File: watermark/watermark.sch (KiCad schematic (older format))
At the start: 7 parts

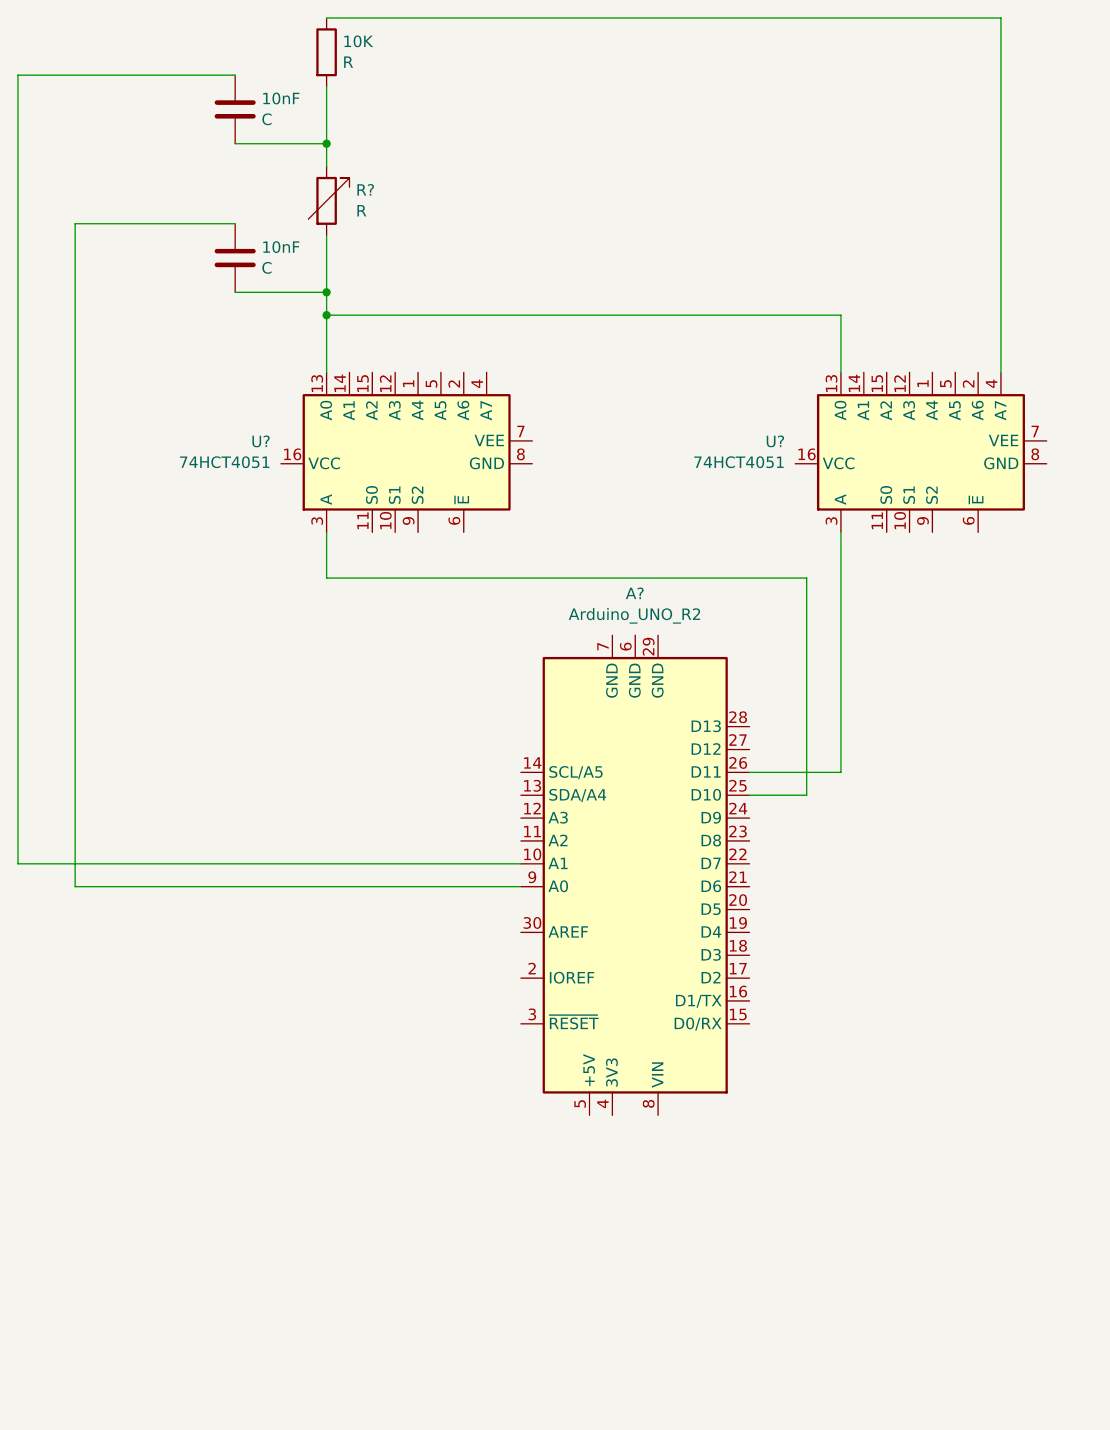
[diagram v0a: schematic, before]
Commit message: m
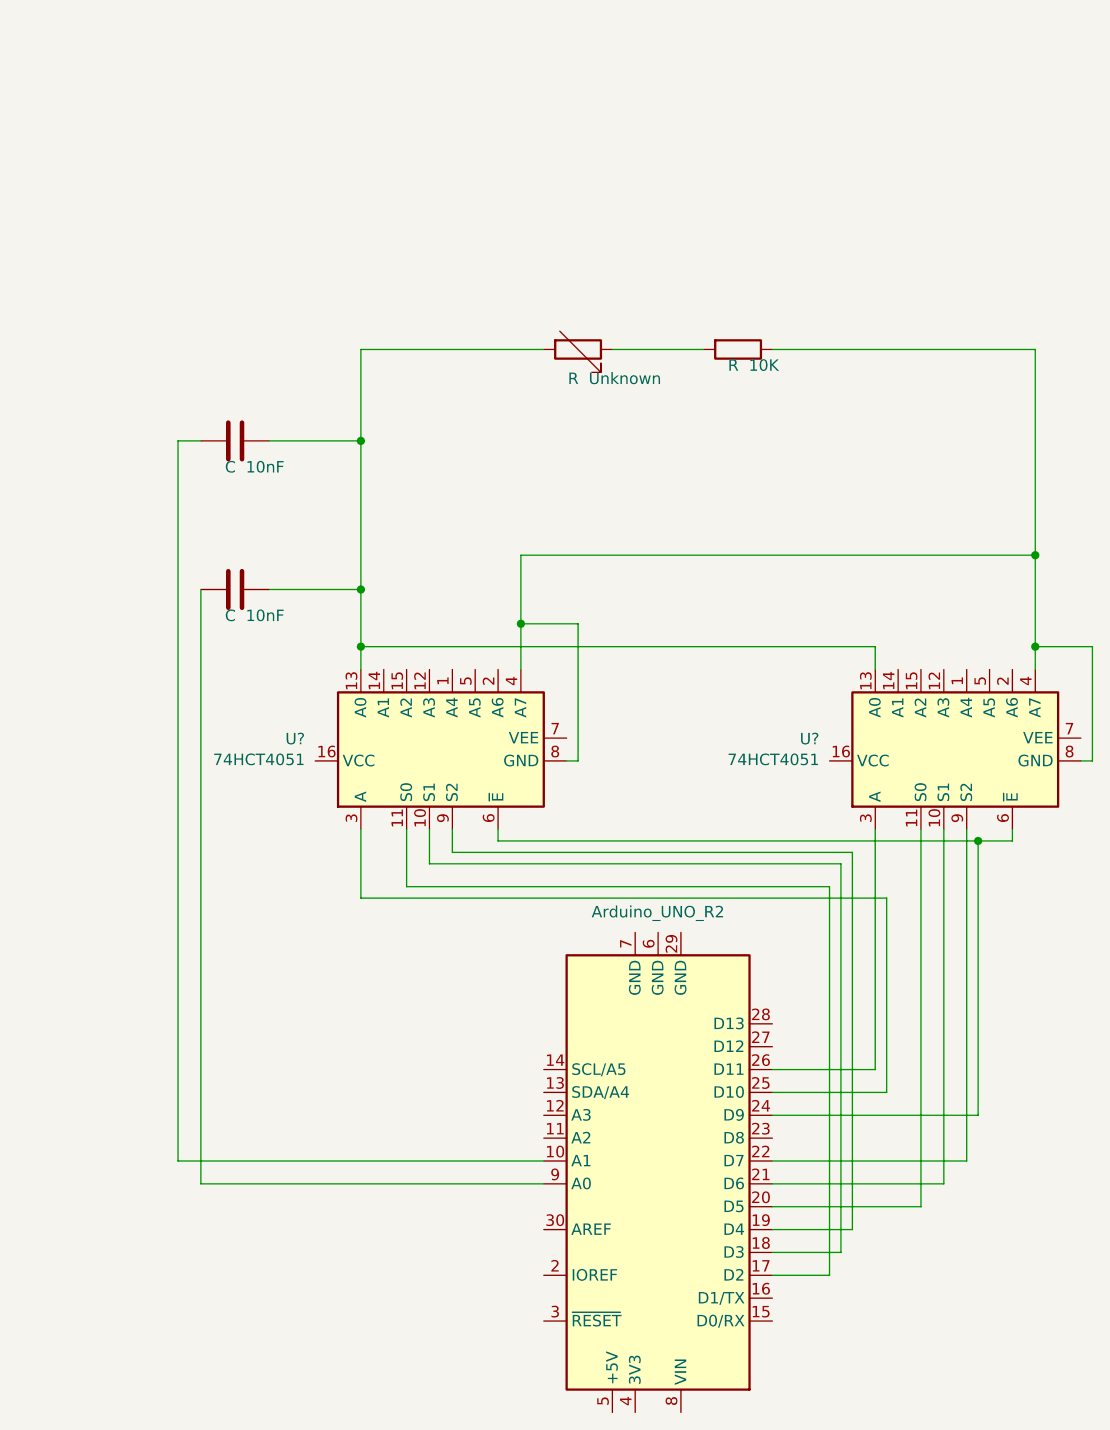
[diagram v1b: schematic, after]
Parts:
- gave numbers to parts that had none: 1
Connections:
- net at U?.10 (S1): now also A?.21 (D6)
- net at U?.11 (S0): now also A?.20 (D5)
- net at U?.13 (A0), U?.13 (A0), Unknown.2: now also 10nF.1, 10nF.1; no longer 10nF.2
- net at 10K.1, U?.4 (A7): now also U?.4 (A7), U?.8 (GND), U?.8 (GND)
- net at U?.6 (~E): now also A?.24 (D9), U?.6 (~E)
- net at U?.9 (S2): now also A?.22 (D7)
- net at U?.10 (S1): now also A?.18 (D3)
- net at U?.11 (S0): now also A?.17 (D2)
- net at U?.9 (S2): now also A?.19 (D4)
- net at 10K.2, Unknown.1: no longer 10nF.2
- net at A?.10 (A1): now also 10nF.2; no longer 10nF.1
- net at A?.9 (A0): now also 10nF.2; no longer 10nF.1
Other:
- moved on the sheet: 10K, 10nF, U?, Unknown
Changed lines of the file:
@@
 $EndDescr
+$Comp
+L Device:R_Variable Unknown
+U 1 1 608B5481
+P 4050 2900
+F 0 "Unknown" V 4178 2946 50  0000 L CNN
+F 1 "R" V 4178 2855 50  0000 L CNN
+F 2 "" V 3980 2900 50  0001 C CNN
+F 3 "~" H 4050 2900 50  0001 C CNN
+	1    4050 2900
+	0    1    1    0
+$EndComp
+$Comp
+L Device:R 10K
+U 1 1 608B5D06
+P 4750 2900
+F 0 "10K" V 4820 2946 50  0000 L CNN
+F 1 "R" V 4820 2855 50  0000 L CNN
+F 2 "" V 4680 2900 50  0001 C CNN
+F 3 "~" H 4750 2900 50  0001 C CNN
+	1    4750 2900
+	0    1    1    0
+$EndComp
+$Comp
+L Device:C 10nF
+U 1 1 608C2E1E
+P 2550 3950
+F 0 "10nF" V 2665 3996 50  0000 L CNN
+F 1 "C" V 2665 3905 50  0000 L CNN
+F 2 "" H 2588 3800 50  0001 C CNN
+F 3 "~" H 2550 3950 50  0001 C CNN
+	1    2550 3950
+	0    1    1    0
+$EndComp
+$Comp
+L Device:C 10nF
+U 1 1 608C5621
+P 2550 3300
+F 0 "10nF" V 2665 3346 50  0000 L CNN
+F 1 "C" V 2665 3255 50  0000 L CNN
+F 2 "" H 2588 3150 50  0001 C CNN
+F 3 "~" H 2550 3300 50  0001 C CNN
+	1    2550 3300
+	0    1    1    0
+$EndComp
+Wire Wire Line
+	3100 5300 3100 5000
+Wire Wire Line
+	3300 5250 3300 5000
+Wire Wire Line
+	3400 5150 3400 5000
+Wire Wire Line
+	5200 5150 3400 5150
+Wire Wire Line
+	4050 4700 4000 4700
+Wire Wire Line
+	5400 5300 3100 5300
+Wire Wire Line
+	5800 5050 5950 5050
+$Comp
+L MCU_Module:Arduino_UNO_R2 A?
+U 1 1 608BD114
+P 4400 6550
+F 0 "A?" H 4400 5269 50  0001 C CNN
+F 1 "Arduino_UNO_R2" H 4400 5361 50  0000 C CNN
+F 2 "Module:Arduino_UNO_R2" H 4400 6550 50  0001 C CIN
+F 3 "https://www.arduino.cc/en/Main/arduinoBoardUno" H 4400 6550 50  0001 C CNN
+	1    4400 6550
+	-1   0    0    1
+$EndComp
+Wire Wire Line
+	4900 6150 5400 6150
+Wire Wire Line
+	5400 6150 5400 5300
+Wire Wire Line
+	4900 6050 5350 6050
+Wire Wire Line
+	5800 5050 5800 6250
+Wire Wire Line
+	4900 6450 5750 6450
+Wire Wire Line
+	4900 6550 5650 6550
+Wire Wire Line
+	4900 6750 5250 6750
+Wire Wire Line
+	4900 6850 5200 6850
+Wire Wire Line
+	5800 6250 4900 6250
+Wire Wire Line
+	5200 6850 5200 5150
+Wire Wire Line
+	5150 5250 3300 5250
+Wire Wire Line
+	4900 6950 5150 6950
+Wire Wire Line
+	5150 6950 5150 5250
+Wire Wire Line
+	5750 6450 5750 5000
+Wire Wire Line
+	5950 5050 5950 5000
+Wire Wire Line
+	5350 6050 5350 5000
+Wire Wire Line
+	5650 6550 5650 5000
 $Comp
 L 74xx:74HCT4051 U?
 U 1 1 608AFB59
-P 5500 3400
-F 0 "U?" V 5596 3944 50  0000 L CNN
-F 1 "74HCT4051" V 5505 3944 50  0000 L CNN
-F 2 "" H 5500 3000 50  0001 C CNN
-F 3 "http://www.ti.com/lit/ds/symlink/cd74hct4051.pdf" H 5500 3000 50  0001 C CNN
-	1    5500 3400
+P 5650 4700
+F 0 "U?" V 5746 5244 50  0000 L CNN
+F 1 "74HCT4051" V 5655 5244 50  0000 L CNN
+F 2 "" H 5650 4300 50  0001 C CNN
+F 3 "http://www.ti.com/lit/ds/symlink/cd74hct4051.pdf" H 5650 4300 50  0001 C CNN
+	1    5650 4700
 	0    -1   -1   0
 $EndComp
+Wire Wire Line
+	5550 5000 5550 6650
+Wire Wire Line
+	5550 6650 4900 6650
 $Comp
 L 74xx:74HCT4051 U?
 U 1 1 608B37CA
-P 3250 3400
-F 0 "U?" V 3346 3944 50  0000 L CNN
-F 1 "74HCT4051" V 3255 3944 50  0000 L CNN
-F 2 "" H 3250 3000 50  0001 C CNN
-F 3 "http://www.ti.com/lit/ds/symlink/cd74hct4051.pdf" H 3250 3000 50  0001 C CNN
-	1    3250 3400
+P 3400 4700
+F 0 "U?" V 3496 5244 50  0000 L CNN
+F 1 "74HCT4051" V 3405 5244 50  0000 L CNN
+F 2 "" H 3400 4300 50  0001 C CNN
+F 3 "http://www.ti.com/lit/ds/symlink/cd74hct4051.pdf" H 3400 4300 50  0001 C CNN
+	1    3400 4700
 	0    -1   -1   0
 $EndComp
-$Comp
-L Device:R_Variable R?
-U 1 1 608B5481
-P 2950 2250
-F 0 "R?" H 3078 2296 50  0000 L CNN
-F 1 "R" H 3078 2205 50  0000 L CNN
-F 2 "" V 2880 2250 50  0001 C CNN
-F 3 "~" H 2950 2250 50  0001 C CNN
-	1    2950 2250
-	1    0    0    -1
-$EndComp
-$Comp
-L Device:R 10K
-U 1 1 608B5D06
-P 2950 1600
-F 0 "10K" H 3020 1646 50  0000 L CNN
-F 1 "R" H 3020 1555 50  0000 L CNN
-F 2 "" V 2880 1600 50  0001 C CNN
-F 3 "~" H 2950 1600 50  0001 C CNN
-	1    2950 1600
-	1    0    0    -1
-$EndComp
-Wire Wire Line
-	2950 3000 2950 2750
-Wire Wire Line
-	2950 2100 2950 2000
-Wire Wire Line
-	2950 1450 5900 1450
-Wire Wire Line
-	5900 1450 5900 3000
-Wire Wire Line
-	5200 3000 5200 2750
-Wire Wire Line
-	5200 2750 2950 2750
-Connection ~ 2950 2750
-$Comp
-L MCU_Module:Arduino_UNO_R2 A?
-U 1 1 608BD114
-P 4300 5250
-F 0 "A?" H 4300 3969 50  0000 C CNN
-F 1 "Arduino_UNO_R2" H 4300 4060 50  0000 C CNN
-F 2 "Module:Arduino_UNO_R2" H 4300 5250 50  0001 C CIN
-F 3 "https://www.arduino.cc/en/Main/arduinoBoardUno" H 4300 5250 50  0001 C CNN
-	1    4300 5250
-	-1   0    0    1
-$EndComp
-Wire Wire Line
-	1850 5250 3800 5250
-Wire Wire Line
-	2950 2000 2550 2000
-Wire Wire Line
-	1600 5150 3800 5150
-Connection ~ 2950 2000
-Wire Wire Line
-	2950 2000 2950 1750
-$Comp
-L Device:C 10nF
-U 1 1 608C2E1E
-P 2550 2500
-F 0 "10nF" H 2665 2546 50  0000 L CNN
-F 1 "C" H 2665 2455 50  0000 L CNN
-F 2 "" H 2588 2350 50  0001 C CNN
-F 3 "~" H 2550 2500 50  0001 C CNN
-	1    2550 2500
-	1    0    0    -1
-$EndComp
-Wire Wire Line
-	2950 2400 2950 2650
-Wire Wire Line
-	2950 2650 2550 2650
-Connection ~ 2950 2650
-Wire Wire Line
-	2950 2650 2950 2750
-Wire Wire Line
-	2550 2350 1850 2350
-Wire Wire Line
-	1850 2350 1850 5250
-$Comp
-L Device:C 10nF
-U 1 1 608C5621
-P 2550 1850
-F 0 "10nF" H 2665 1896 50  0000 L CNN
-F 1 "C" H 2665 1805 50  0000 L CNN
-F 2 "" H 2588 1700 50  0001 C CNN
-F 3 "~" H 2550 1850 50  0001 C CNN
-	1    2550 1850
-	1    0    0    -1
-$EndComp
-Wire Wire Line
-	2550 1700 1600 1700
-Wire Wire Line
-	1600 1700 1600 5150
-Wire Wire Line
-	5050 3900 2950 3900
-Wire Wire Line
-	2950 3900 2950 3700
-Wire Wire Line
-	4800 4850 5050 4850
-Wire Wire Line
-	5050 4850 5050 3900
-Wire Wire Line
-	4800 4750 5200 4750
-Wire Wire Line
-	5200 4750 5200 3700
+Wire Wire Line
+	5250 6750 5250 5100
+Wire Wire Line
+	5250 5100 3500 5100
+Wire Wire Line
+	3500 5100 3500 5000
+Wire Wire Line
+	3700 5000 3700 5050
+Wire Wire Line
+	3700 5050 5800 5050
+Connection ~ 5800 5050
+Wire Wire Line
+	2400 3950 2400 6550
+Wire Wire Line
+	2400 6550 3900 6550
+Wire Wire Line
+	2400 3300 2300 3300
+Wire Wire Line
+	2300 3300 2300 6450
+Wire Wire Line
+	2300 6450 3900 6450
+Wire Wire Line
+	3100 2900 3900 2900
+Wire Wire Line
+	4200 2900 4600 2900
+Wire Wire Line
+	3100 3300 2700 3300
+Connection ~ 3100 3300
+Wire Wire Line
+	3100 3300 3100 2900
+Connection ~ 3100 3950
+Wire Wire Line
+	3100 3950 3100 3300
+Wire Wire Line
+	5350 4300 5350 4200
+Wire Wire Line
+	6050 3800 3800 3800
+Wire Wire Line
+	3800 3800 3800 4100
+Wire Wire Line
+	6050 3800 6050 4200
+Wire Wire Line
+	5350 4200 3100 4200
+Wire Wire Line
+	3100 3950 3100 4200
+Connection ~ 3100 4200
+Wire Wire Line
+	3100 4200 3100 4300
+Wire Wire Line
+	2700 3950 3100 3950
+Wire Wire Line
+	4900 2900 6050 2900
+Wire Wire Line
+	6050 2900 6050 3800
+Connection ~ 6050 3800
+Wire Wire Line
+	3800 4100 4050 4100
+Wire Wire Line
+	4050 4100 4050 4700
+Connection ~ 3800 4100
+Wire Wire Line
+	3800 4100 3800 4300
+Wire Wire Line
+	6250 4700 6300 4700
+Wire Wire Line
+	6300 4700 6300 4200
+Wire Wire Line
+	6300 4200 6050 4200
+Connection ~ 6050 4200
+Wire Wire Line
+	6050 4200 6050 4300
 $EndSCHEMATC
